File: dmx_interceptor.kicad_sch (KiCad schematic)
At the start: 8 parts, among them J1 TB010-508-02BE, J2 TB010-508-02BE, J3 TB004-508-03BE, J4 TB004-508-03BE, U1 ARDUINO_PRO_MINI

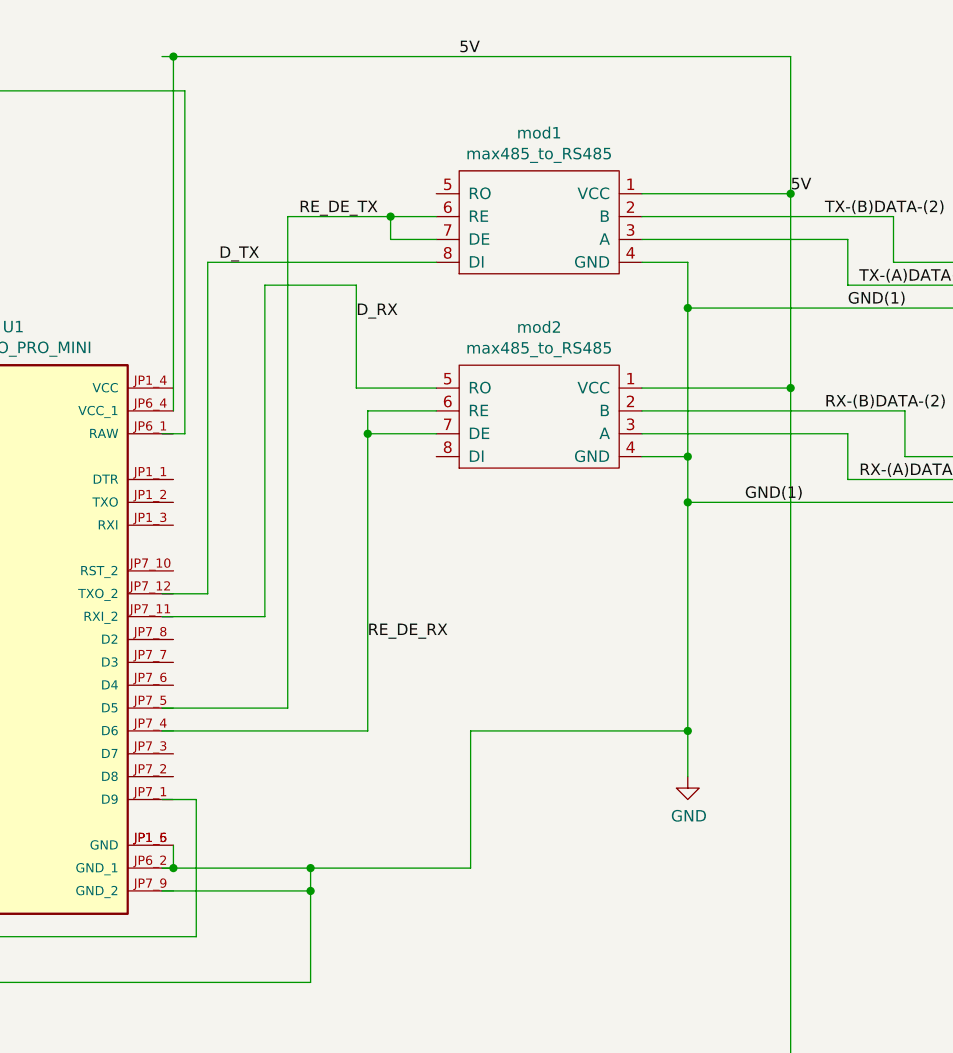
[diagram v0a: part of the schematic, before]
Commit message: output files for ordering & pcb fix
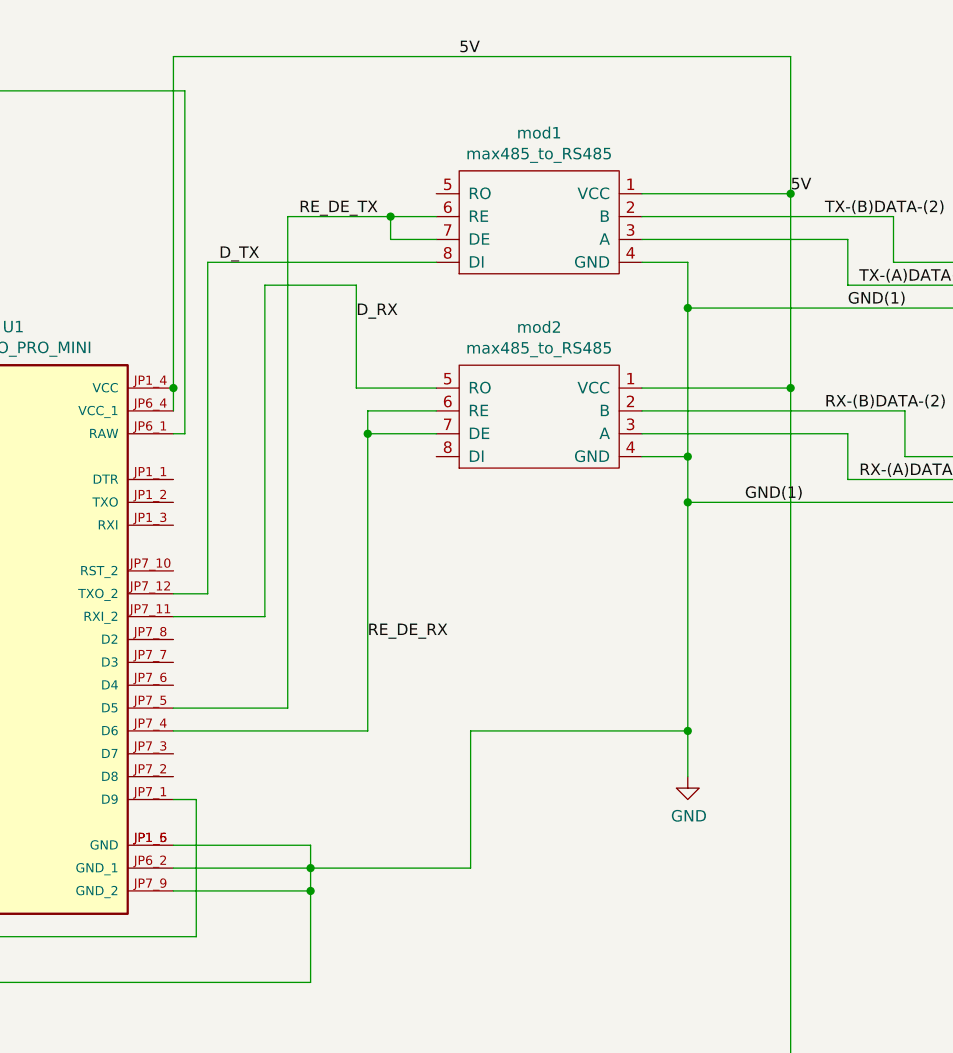
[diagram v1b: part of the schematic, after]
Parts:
- J1, J2: footprint CUI_TB010-508-02BE -> dmx_interceptor:CUI_TB010-508-02BE; MPN (none) -> TB010-508-02BE
- J3, J4: footprint CUI_TB004-508-03BE -> dmx_interceptor:CUI_TB004-508-03BE; MPN (none) -> TB004-508-03BE
- R1: footprint mart_library:smd_0603_1608-Metric -> dmx_interceptor:smd_0603_1608-Metric
- U1: footprint MODULE_ARDUINO_PRO_MINI -> dmx_interceptor:MODULE_ARDUINO_PRO_MINI; MPN (none) -> DEV-11113
- mod1, mod2: footprint mart_library:max485_to_rs485 -> dmx_interceptor:max485_to_rs485
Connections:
- net 5V: now also U1.JP1_4 (VCC)
- net D_RX: now also U1.JP7_11 (RXI_2)
- net D_TX: now also U1.JP7_12 (TXO_2)
- net GND: now also U1.JP7_9 (GND_2)
- net RE_DE_RX: now also U1.JP7_4 (D6)
- net RE_DE_TX: now also U1.JP7_5 (D5)
- net VIN: now also U1.JP6_1 (RAW)
- net switch: now also U1.JP7_1 (D9)
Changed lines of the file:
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@@
 (kicad_sch (version 20230121) (generator eeschema)
   (paper "A4")
+  (junction (at 143.51 66.04) (diameter 0) (color 0 0 0 0)
+  )
   (junction (at 200.66 73.66) (diameter 0) (color 0 0 0 0)
   )
+  (junction (at 158.75 119.38) (diameter 0) (color 0 0 0 0)
+  )
   (junction (at 212.09 66.04) (diameter 0) (color 0 0 0 0)
   )
-  (junction (at 158.75 119.38) (diameter 0) (color 0 0 0 0)
-  )
-  (junction (at 143.51 29.21) (diameter 0) (color 0 0 0 0)
+  (junction (at 158.75 121.92) (diameter 0) (color 0 0 0 0)
   )
   (junction (at 167.64 46.99) (diameter 0) (color 0 0 0 0)
@@
   (junction (at 200.66 104.14) (diameter 0) (color 0 0 0 0)
   )
-  (junction (at 143.51 119.38) (diameter 0) (color 0 0 0 0)
-  )
   (junction (at 165.1 71.12) (diameter 0) (color 0 0 0 0)
   )
@@
   (junction (at 200.66 57.15) (diameter 0) (color 0 0 0 0)
   )
-  (junction (at 158.75 121.92) (diameter 0) (color 0 0 0 0)
-  )
   (wire (pts (xy 153.67 91.44) (xy 153.67 54.61))
     (stroke (width 0) (type default))
@@
     (stroke (width 0) (type default))
   )
+  (wire (pts (xy 143.51 29.21) (xy 143.51 66.04))
+    (stroke (width 0) (type default))
+  )
   (wire (pts (xy 212.09 66.04) (xy 195.58 66.04))
     (stroke (width 0) (type default))
@@
     (stroke (width 0) (type default))
   )
-  (wire (pts (xy 142.24 91.44) (xy 153.67 91.44))
-    (stroke (width 0) (type default))
-  )
   (wire (pts (xy 200.66 109.22) (xy 200.66 104.14))
     (stroke (width 0) (type default))
@@
     (stroke (width 0) (type default))
   )
-  (wire (pts (xy 143.51 119.38) (xy 142.24 119.38))
+  (wire (pts (xy 143.51 121.92) (xy 158.75 121.92))
+    (stroke (width 0) (type default))
+  )
+  (wire (pts (xy 143.51 91.44) (xy 153.67 91.44))
     (stroke (width 0) (type default))
   )
@@
     (stroke (width 0) (type default))
   )
-  (wire (pts (xy 143.51 29.21) (xy 143.51 68.58))
+  (wire (pts (xy 143.51 66.04) (xy 143.51 68.58))
     (stroke (width 0) (type default))
   )
@@
     (stroke (width 0) (type default))
   )
-  (wire (pts (xy 212.09 29.21) (xy 143.51 29.21))
+  (wire (pts (xy 143.51 101.6) (xy 156.21 101.6))
+    (stroke (width 0) (type default))
+  )
+  (wire (pts (xy 143.51 116.84) (xy 158.75 116.84))
     (stroke (width 0) (type default))
   )
@@
     (stroke (width 0) (type default))
   )
-  (wire (pts (xy 142.24 71.12) (xy 144.78 71.12))
-    (stroke (width 0) (type default))
-  )
   (wire (pts (xy 125.73 153.67) (xy 212.09 153.67))
     (stroke (width 0) (type default))
@@
     (stroke (width 0) (type default))
   )
-  (wire (pts (xy 142.24 104.14) (xy 165.1 104.14))
+  (wire (pts (xy 143.51 29.21) (xy 212.09 29.21))
+    (stroke (width 0) (type default))
+  )
+  (wire (pts (xy 158.75 116.84) (xy 158.75 119.38))
+    (stroke (width 0) (type default))
+  )
+  (wire (pts (xy 143.51 111.76) (xy 146.05 111.76))
     (stroke (width 0) (type default))
   )
@@
     (stroke (width 0) (type default))
   )
+  (wire (pts (xy 143.51 104.14) (xy 165.1 104.14))
+    (stroke (width 0) (type default))
+  )
   (wire (pts (xy 92.71 127) (xy 146.05 127))
     (stroke (width 0) (type default))
   )
-  (wire (pts (xy 142.24 88.9) (xy 147.32 88.9))
+  (wire (pts (xy 143.51 119.38) (xy 158.75 119.38))
     (stroke (width 0) (type default))
   )
@@
     (stroke (width 0) (type default))
   )
-  (wire (pts (xy 143.51 29.21) (xy 142.24 29.21))
+  (wire (pts (xy 143.51 88.9) (xy 147.32 88.9))
     (stroke (width 0) (type default))
   )
@@
     (stroke (width 0) (type default))
   )
-  (wire (pts (xy 142.24 121.92) (xy 158.75 121.92))
-    (stroke (width 0) (type default))
-  )
   (wire (pts (xy 153.67 54.61) (xy 163.83 54.61))
     (stroke (width 0) (type default))
@@
     (stroke (width 0) (type default))
   )
-  (wire (pts (xy 158.75 119.38) (xy 143.51 119.38))
-    (stroke (width 0) (type default))
-  )
-  (wire (pts (xy 142.24 101.6) (xy 156.21 101.6))
-    (stroke (width 0) (type default))
-  )
   (wire (pts (xy 165.1 71.12) (xy 172.72 71.12))
     (stroke (width 0) (type default))
   )
+  (wire (pts (xy 143.51 71.12) (xy 144.78 71.12))
+    (stroke (width 0) (type default))
+  )
   (wire (pts (xy 195.58 44.45) (xy 212.09 44.45))
     (stroke (width 0) (type default))
@@
     (stroke (width 0) (type default))
   )
-  (wire (pts (xy 158.75 121.92) (xy 158.75 119.38))
+  (wire (pts (xy 158.75 119.38) (xy 158.75 121.92))
     (stroke (width 0) (type default))
   )
@@
     (stroke (width 0) (type default))
   )
+  (wire (pts (xy 200.66 104.14) (xy 176.53 104.14))
+    (stroke (width 0) (type default))
+  )
+  (wire (pts (xy 212.09 44.45) (xy 212.09 29.21))
+    (stroke (width 0) (type default))
+  )
+  (wire (pts (xy 200.66 57.15) (xy 200.66 73.66))
+    (stroke (width 0) (type default))
+  )
+  (wire (pts (xy 66.04 109.22) (xy 53.34 109.22))
+    (stroke (width 0) (type default))
+  )
+  (wire (pts (xy 218.44 49.53) (xy 218.44 54.61))
+    (stroke (width 0) (type default))
+  )
+  (wire (pts (xy 172.72 68.58) (xy 165.1 68.58))
+    (stroke (width 0) (type default))
+  )
+  (wire (pts (xy 158.75 132.08) (xy 86.36 132.08))
+    (stroke (width 0) (type default))
+  )
+  (wire (pts (xy 156.21 46.99) (xy 156.21 101.6))
+    (stroke (width 0) (type default))
+  )
   (wire (pts (xy 158.75 121.92) (xy 158.75 132.08))
     (stroke (width 0) (type default))
   )
-  (wire (pts (xy 200.66 104.14) (xy 176.53 104.14))
-    (stroke (width 0) (type default))
-  )
-  (wire (pts (xy 143.51 116.84) (xy 143.51 119.38))
-    (stroke (width 0) (type default))
-  )
-  (wire (pts (xy 212.09 44.45) (xy 212.09 29.21))
-    (stroke (width 0) (type default))
-  )
-  (wire (pts (xy 200.66 57.15) (xy 200.66 73.66))
-    (stroke (width 0) (type default))
-  )
-  (wire (pts (xy 66.04 109.22) (xy 53.34 109.22))
-    (stroke (width 0) (type default))
-  )
-  (wire (pts (xy 218.44 49.53) (xy 218.44 54.61))
-    (stroke (width 0) (type default))
-  )
-  (wire (pts (xy 172.72 68.58) (xy 165.1 68.58))
-    (stroke (width 0) (type default))
-  )
-  (wire (pts (xy 158.75 132.08) (xy 86.36 132.08))
-    (stroke (width 0) (type default))
-  )
-  (wire (pts (xy 156.21 46.99) (xy 156.21 101.6))
-    (stroke (width 0) (type default))
-  )
   (wire (pts (xy 77.47 33.02) (xy 144.78 33.02))
     (stroke (width 0) (type default))
   )
   (wire (pts (xy 200.66 73.66) (xy 195.58 73.66))
-    (stroke (width 0) (type default))
-  )
-  (wire (pts (xy 142.24 111.76) (xy 146.05 111.76))
     (stroke (width 0) (type default))
   )
@@
       (effects (font (size 1.27 1.27)) (justify left))
     )
-    (property "Footprint" "CUI_TB004-508-03BE" (at 242.57 54.61 0)
+    (property "Footprint" "dmx_interceptor:CUI_TB004-508-03BE" (at 242.57 54.61 0)
       (effects (font (size 1.27 1.27)) (justify left bottom) hide)
     )
@@
     )
     (property "mpn" "TB004-508-03BE" (at 248.92 39.37 0)
+      (effects (font (size 1.27 1.27)) hide)
+    )
+    (property "MPN" "TB004-508-03BE" (at 242.57 54.61 0)
       (effects (font (size 1.27 1.27)) hide)
     )
@@
       (effects (font (size 1.27 1.27)) (justify left))
     )
-    (property "Footprint" "CUI_TB004-508-03BE" (at 242.57 76.2 0)
+    (property "Footprint" "dmx_interceptor:CUI_TB004-508-03BE" (at 242.57 76.2 0)
       (effects (font (size 1.27 1.27)) (justify left bottom) hide)
     )
@@
     )
     (property "mpn" "TB004-508-03BE" (at 248.92 60.96 0)
+      (effects (font (size 1.27 1.27)) hide)
+    )
+    (property "MPN" "TB004-508-03BE" (at 242.57 76.2 0)
       (effects (font (size 1.27 1.27)) hide)
     )
@@
       (effects (font (size 1.27 1.27)))
     )
-    (property "Footprint" "CUI_TB010-508-02BE" (at 115.57 153.67 0)
+    (property "Footprint" "dmx_interceptor:CUI_TB010-508-02BE" (at 115.57 153.67 0)
       (effects (font (size 1.27 1.27)) (justify left bottom) hide)
     )
@@
     )
     (property "mnp" "TB010-508-02BE" (at 115.57 153.67 0)
+      (effects (font (size 1.27 1.27)) hide)
+    )
+    (property "MPN" "TB010-508-02BE" (at 115.57 153.67 0)
       (effects (font (size 1.27 1.27)) hide)
     )
@@
       (effects (font (size 1.27 1.27)) hide)
     )
-    (property "Footprint" "mart_library:smd_0603_1608-Metric" (at 69.85 103.632 90)
+    (property "Footprint" "dmx_interceptor:smd_0603_1608-Metric" (at 69.85 103.632 90)
       (effects (font (size 1.27 1.27)) hide)
     )
@@
       (effects (font (size 1.27 1.27)))
     )
-    (property "Footprint" "mart_library:max485_to_rs485" (at 181.61 63.5 0)
+    (property "Footprint" "dmx_interceptor:max485_to_rs485" (at 181.61 63.5 0)
       (effects (font (size 1.27 1.27)) hide)
     )
@@
       (effects (font (size 1.27 1.27)))
     )
-    (property "Footprint" "mart_library:max485_to_rs485" (at 181.61 85.09 0)
+    (property "Footprint" "dmx_interceptor:max485_to_rs485" (at 181.61 85.09 0)
       (effects (font (size 1.27 1.27)) hide)
     )
@@
       (effects (font (size 1.27 1.27)))
     )
-    (property "Footprint" "CUI_TB010-508-02BE" (at 67.31 33.02 0)
+    (property "Footprint" "dmx_interceptor:CUI_TB010-508-02BE" (at 67.31 33.02 0)
       (effects (font (size 1.27 1.27)) (justify left bottom) hide)
     )
@@
     )
     (property "mnp" "TB010-508-02BE" (at 67.31 33.02 0)
+      (effects (font (size 1.27 1.27)) hide)
+    )
+    (property "MPN" "TB010-508-02BE" (at 67.31 33.02 0)
       (effects (font (size 1.27 1.27)) hide)
     )
@@
       (effects (font (size 1.27 1.27)))
     )
-    (property "Footprint" "MODULE_ARDUINO_PRO_MINI" (at 125.73 93.98 0)
+    (property "Footprint" "dmx_interceptor:MODULE_ARDUINO_PRO_MINI" (at 125.73 93.98 0)
       (effects (font (size 1.27 1.27)) (justify left bottom) hide)
     )
@@
       (effects (font (size 1.27 1.27)) hide)
     )
+    (property "MPN" "DEV-11113" (at 125.73 93.98 0)
+      (effects (font (size 1.27 1.27)) hide)
+    )
